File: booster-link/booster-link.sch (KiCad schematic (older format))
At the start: 28 parts, among them P1 Conn_01x04, P2 IBT-2, P3 EXTCON, P4 CONN_01X03, Q1 BC517, Q21 BC517, U1 7805, U11 TLC555CP, U2 6N137

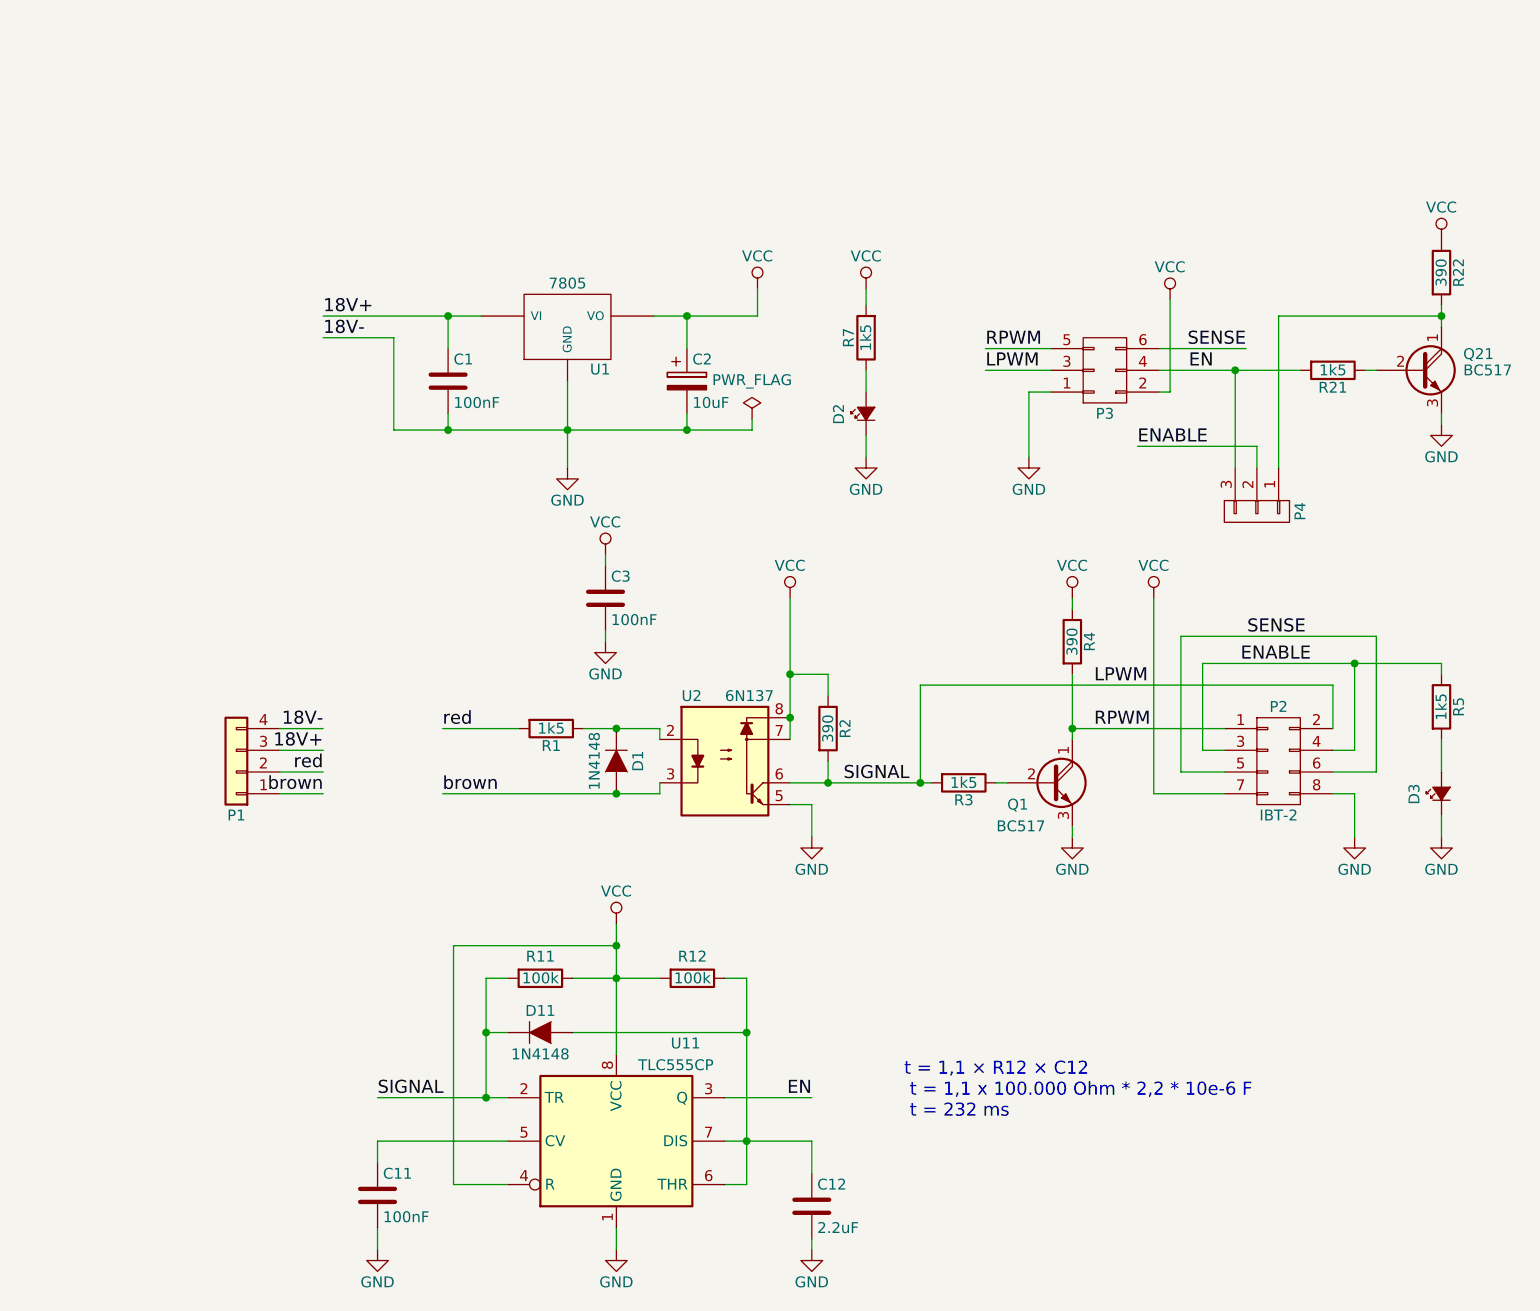
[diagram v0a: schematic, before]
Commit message: wip
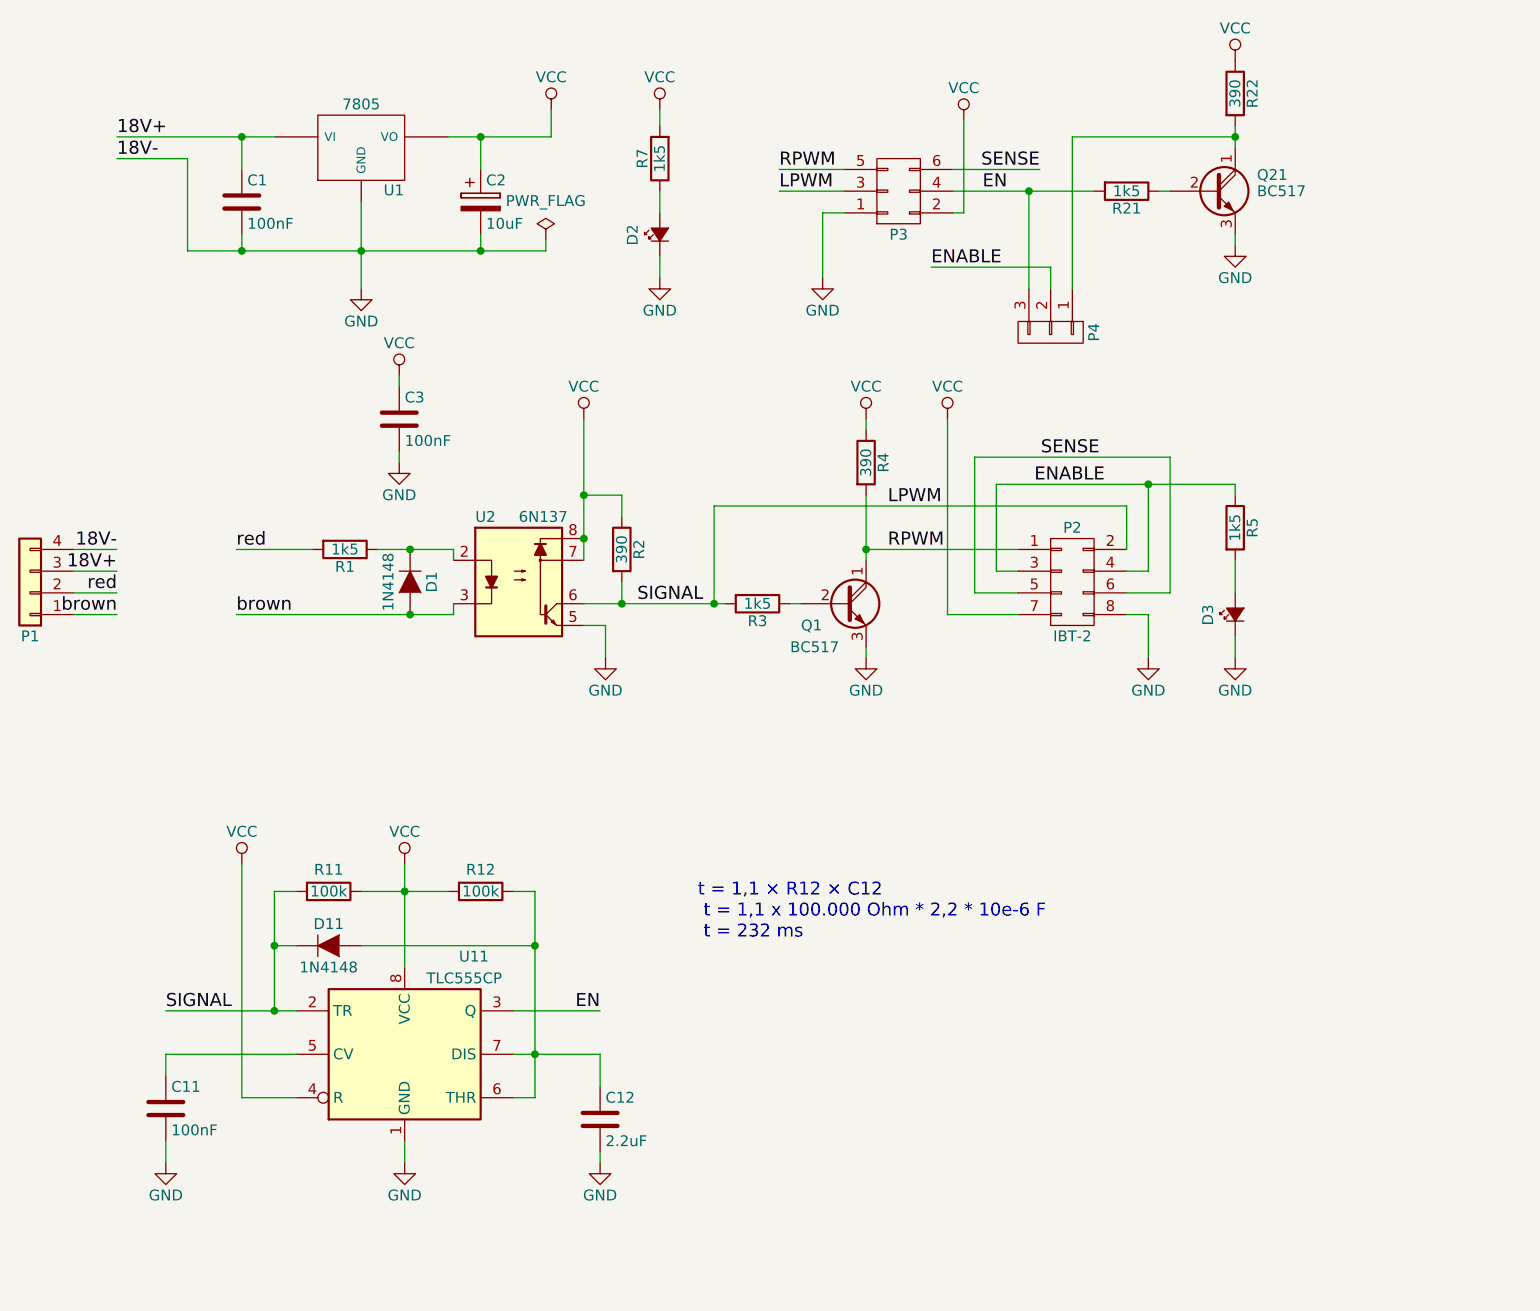
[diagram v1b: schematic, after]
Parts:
- D2, D3: footprint LEDs:LED-5MM -> LEDs:LED_D5.0mm
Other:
- moved on the sheet: C1, C11, C12, C2, C3, D1, D11, D2, D3, P1, P2, P3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
